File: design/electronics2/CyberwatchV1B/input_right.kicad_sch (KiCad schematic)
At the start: 3 parts, among them J8 Conn_01x07_IR_main, SW4 SW_Push, U5 MT6701CT

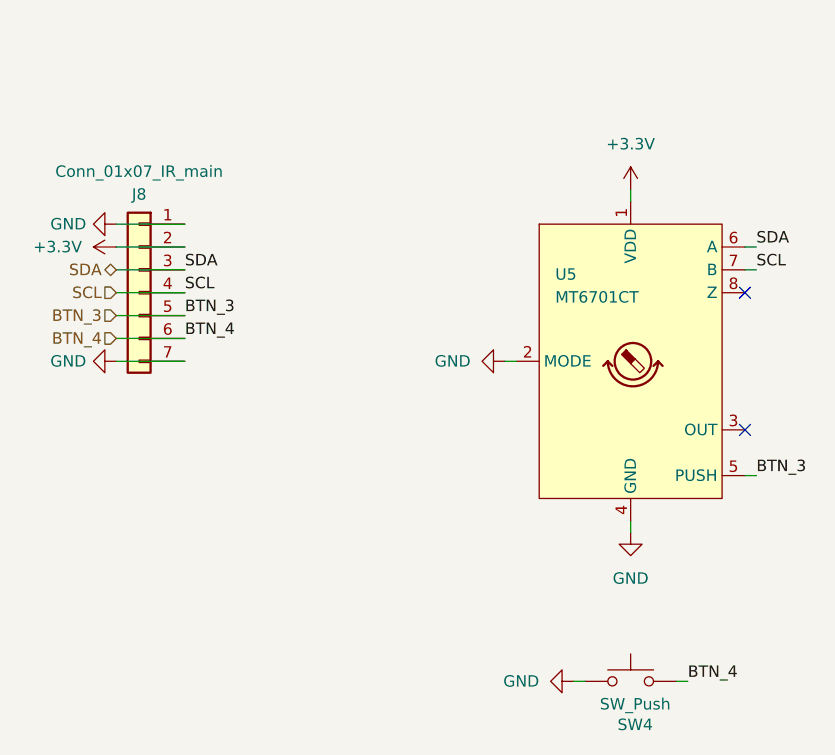
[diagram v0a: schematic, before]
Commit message: pcb design
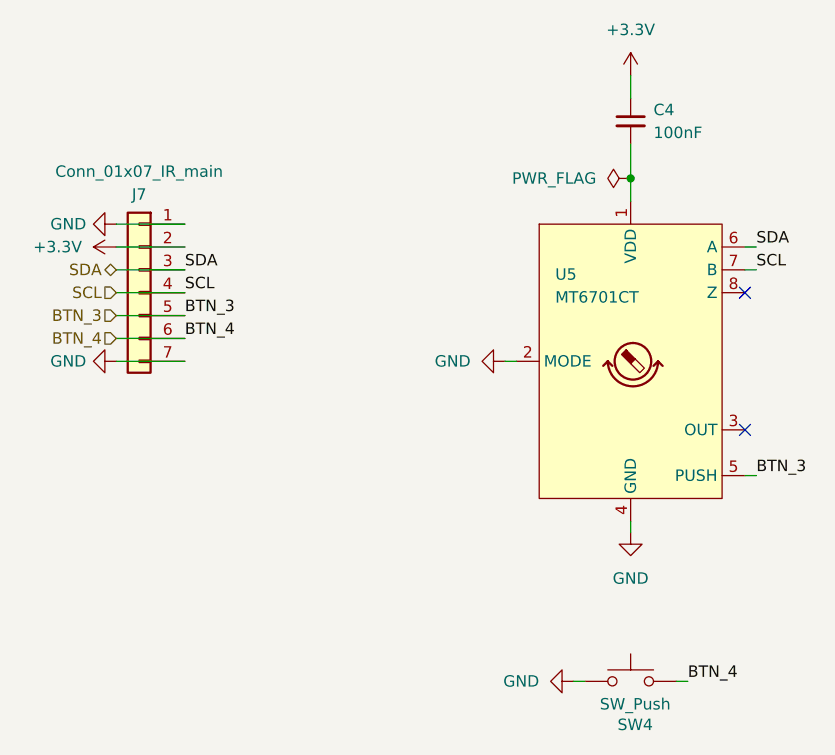
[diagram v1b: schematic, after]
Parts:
- added C4: 100nF, Capacitor_SMD:C_0603_1608Metric, symbol Device:C_Small
- J7: renamed from J8; KiLib_Generator (none) -> connector/SMD_single_row_plus_mounting_pad
- U5: KiLib_Generator (none) -> package/gullwing
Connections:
- net +3.3V: now also C4.1; no longer U5.1 (VDD)
- new net: C4.2, U5.1 (VDD)

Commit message: PCB design finalisation
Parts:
- C4: MPN (none) -> CL10B104KB8NNNC
- J7: MPN (none) -> SM07B-SRSS-TB(LF)(SN)
- SW4: MPN (none) -> KMR231NG LFS
- U5: MPN (none) -> MT6701CT-STD
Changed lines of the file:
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@@
+			)
+		)
+		(property "MPN" "MT6701CT-STD"
+			(at 134.62 66.04 0)
+			(hide yes)
+			(show_name no)
+			(do_not_autoplace no)
+			(effects
+				(font
+					(size 1.27 1.27)
+				)
 			)
 		)
@@
 			)
 		)
+		(property "MPN" " SM07B-SRSS-TB(LF)(SN)"
+			(at 80.01 58.42 0)
+			(hide yes)
+			(show_name no)
+			(do_not_autoplace no)
+			(effects
+				(font
+					(size 1.27 1.27)
+				)
+			)
+		)
 		(pin "2"
 		)
@@
 			)
 		)
+		(property "MPN" "CL10B104KB8NNNC"
+			(at 134.62 39.37 0)
+			(hide yes)
+			(show_name no)
+			(do_not_autoplace no)
+			(effects
+				(font
+					(size 1.27 1.27)
+				)
+			)
+		)
 		(pin "1"
 		)
@@
 			(at 134.62 101.6 0)
 			(hide yes)
+			(show_name no)
+			(do_not_autoplace no)
+			(effects
+				(font
+					(size 1.27 1.27)
+				)
+			)
+		)
+		(property "MPN" " KMR231NG LFS"
+			(at 134.62 101.6 0)
+			(hide yes)
